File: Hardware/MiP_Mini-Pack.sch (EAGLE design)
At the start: 41 parts, among them Q1 8MHz, U1 ATMEGA328, U3 TS3USB221A

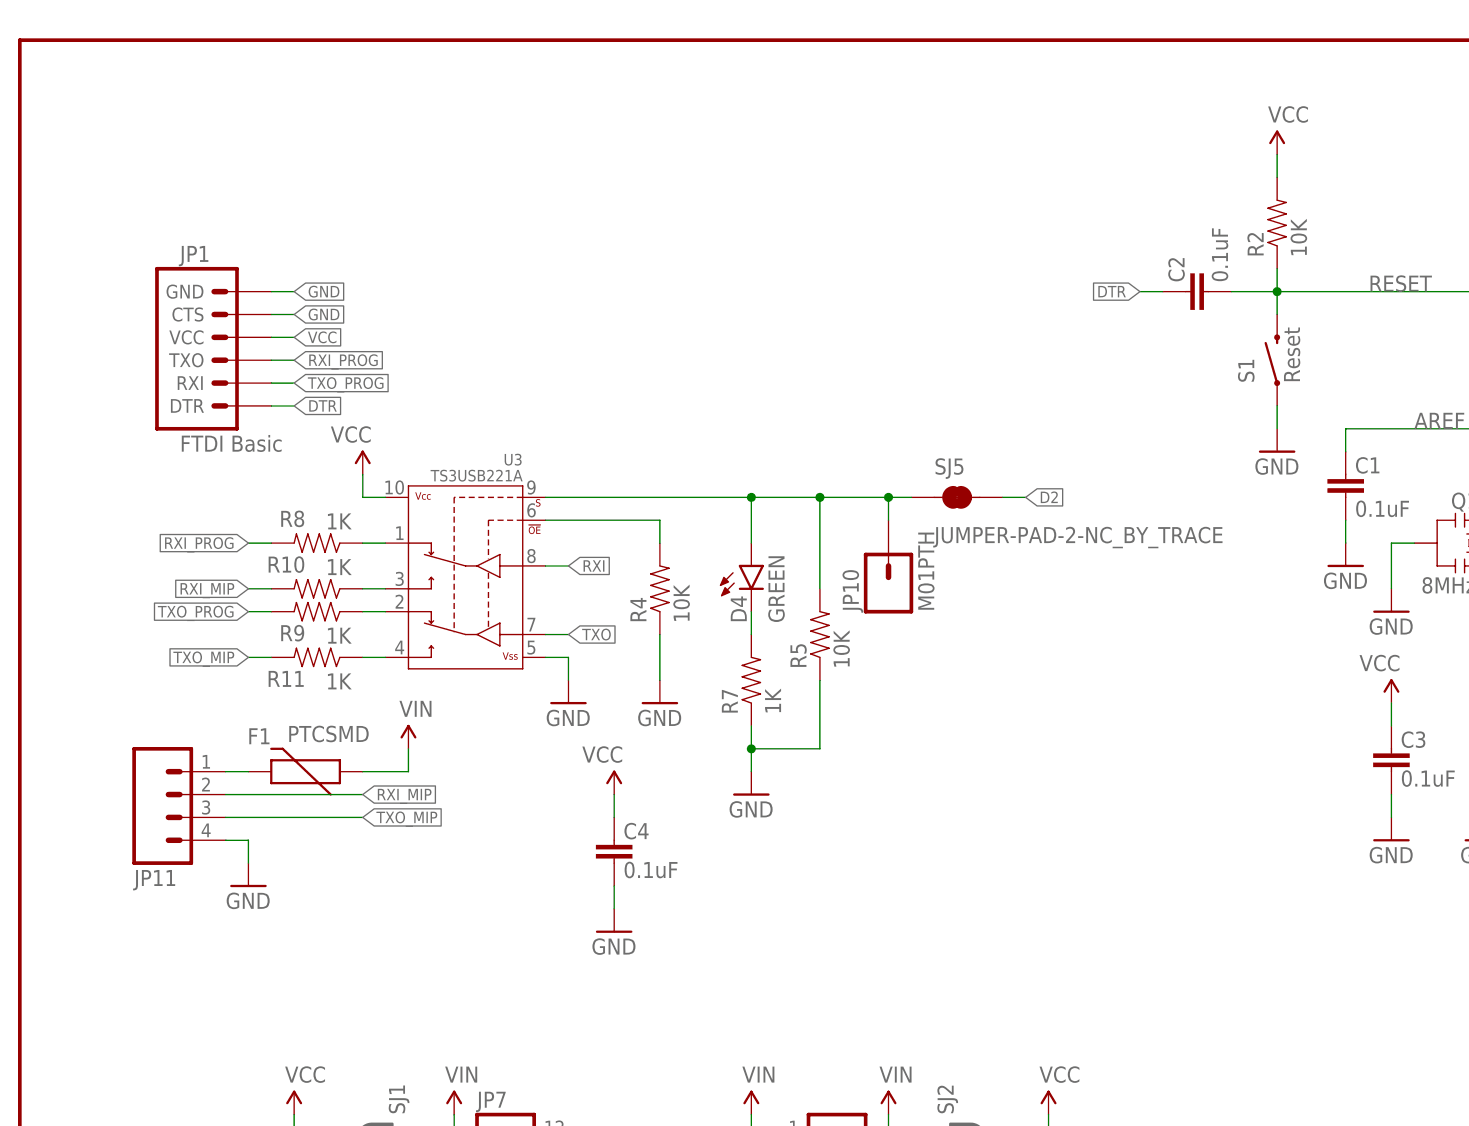
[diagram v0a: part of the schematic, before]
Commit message: corrected labels, ready for review
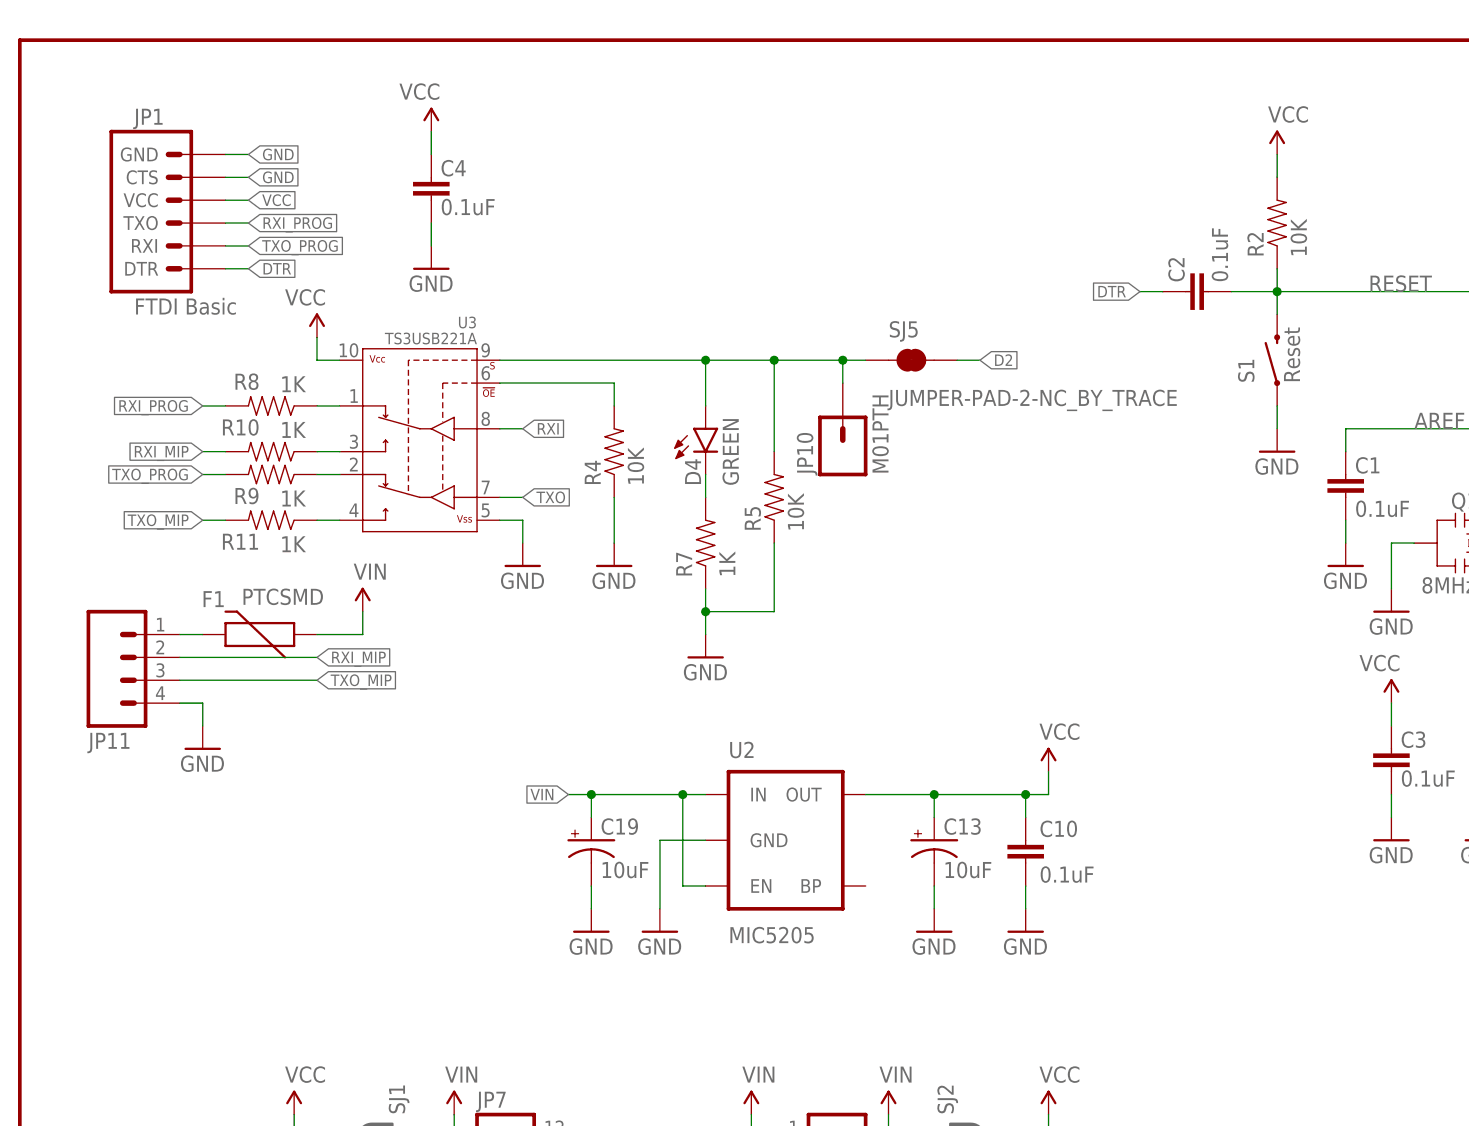
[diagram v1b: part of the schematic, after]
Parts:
- added C10: 0.1uF, SparkFun:CAP0603-CAP
- added C13, C19: 10uF, SparkFun:CAP_POL1206
- added U2: MIC5205, SparkFun:V_REG_LDOSMD
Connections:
- net GND: now also C10.2, C13.-, C19.-, U2.GND
- net VCC: now also C10.1, C13.+, U2.OUT
- net VIN: now also C19.+, U2.EN, U2.IN
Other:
- moved on the sheet: C4, D4, F1, JP1, JP10, JP11, R10, R11, R4, R5, R7, R8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
